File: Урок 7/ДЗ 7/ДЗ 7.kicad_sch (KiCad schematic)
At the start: 22 parts, among them SW1 SW_Push, SW2 SW_Push

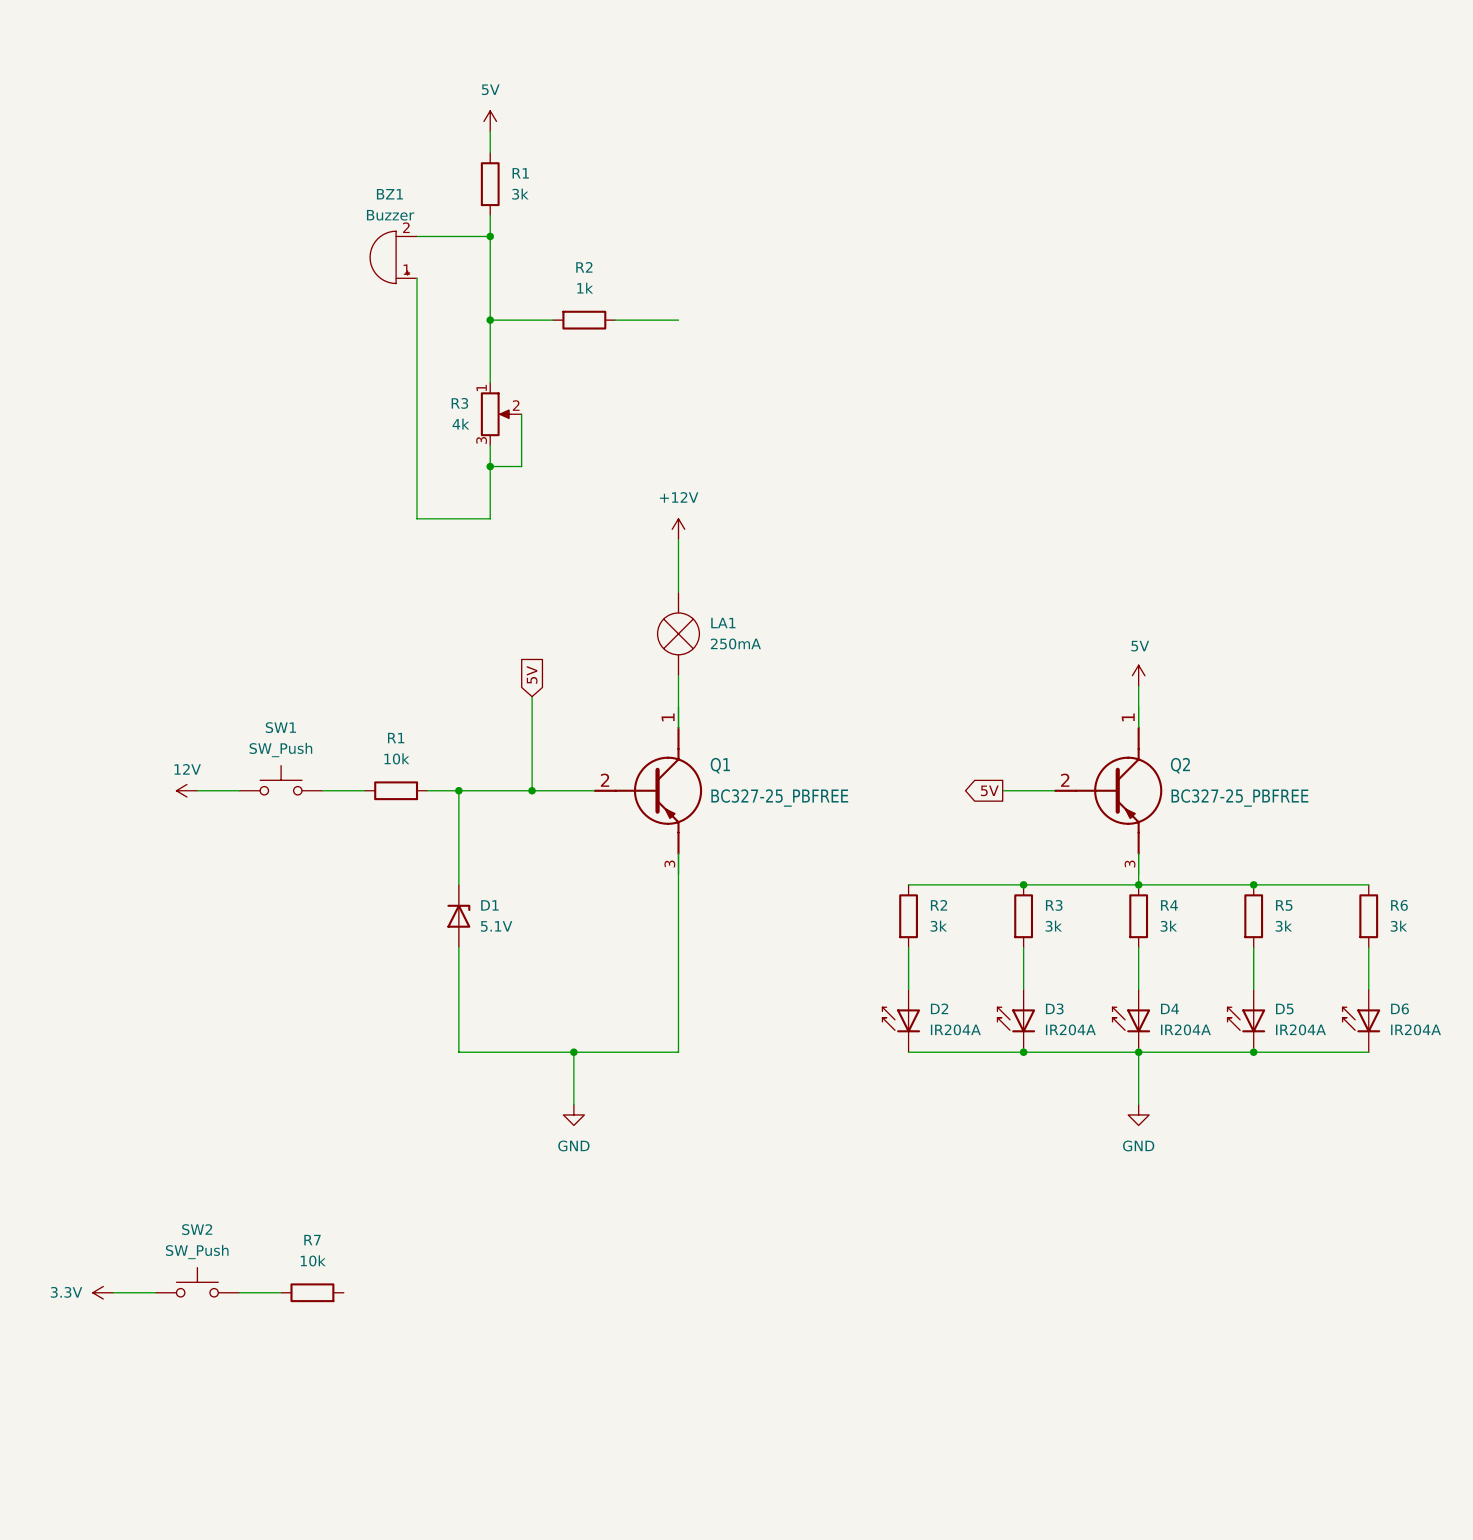
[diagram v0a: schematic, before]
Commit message: 1
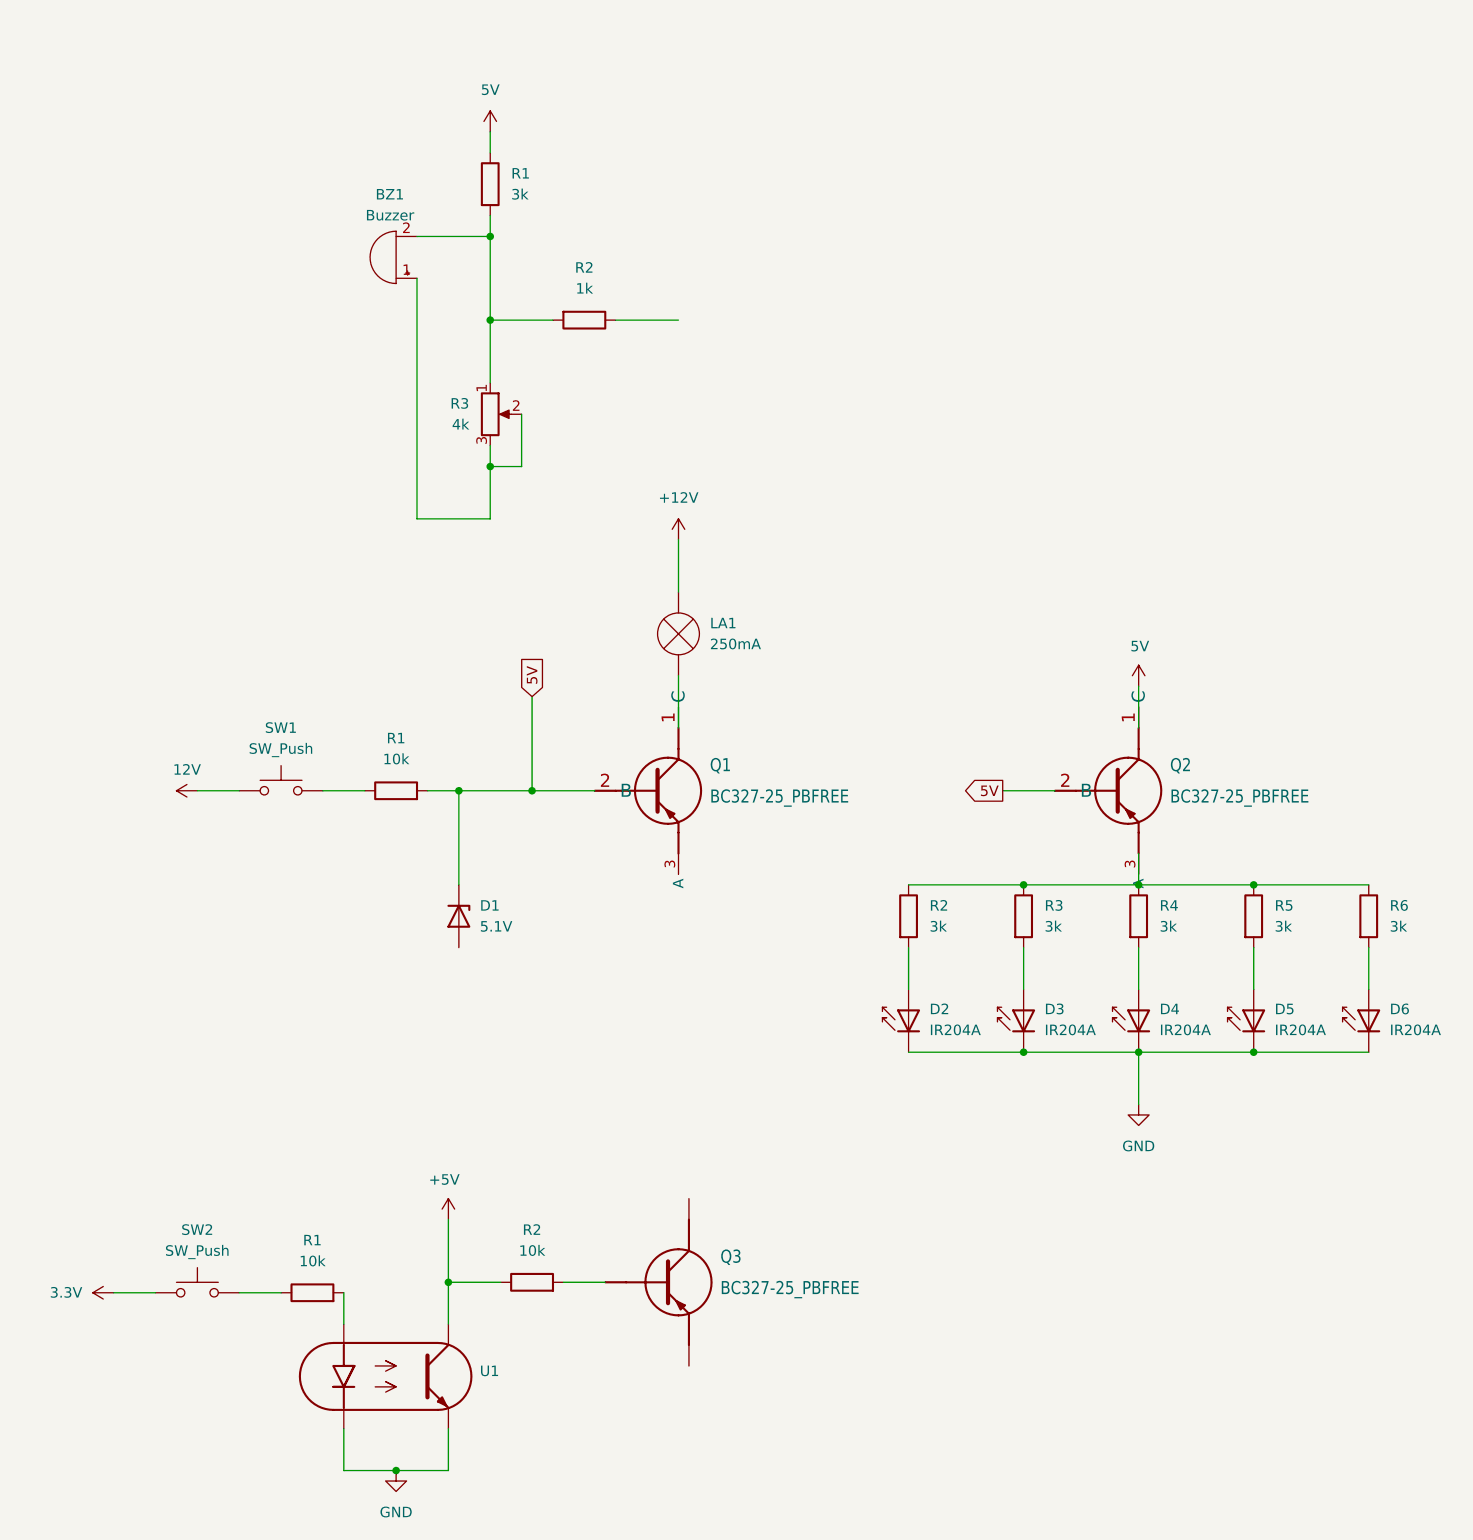
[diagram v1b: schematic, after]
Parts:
- added Q3: ~, cadstarpcblib:BC32725PBFREE, symbol My_lib2:BC327-25_PBFREE
- added R2: 10k, symbol Device:R
- added U1: ~, symbol My_lib2:PC817X3NSZ9F
- renumbered R7 to R1
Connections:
- net GND: now also U1.2 (Cathode), U1.3 (Emitter); no longer D1.2 (A), Q1.3 (A)
- net at R1.2: now also U1.1 (Anode)
- new net: Q3.2 (B), R2.2
- new net +5V: R2.1, U1.4 (Collector)

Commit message: 1
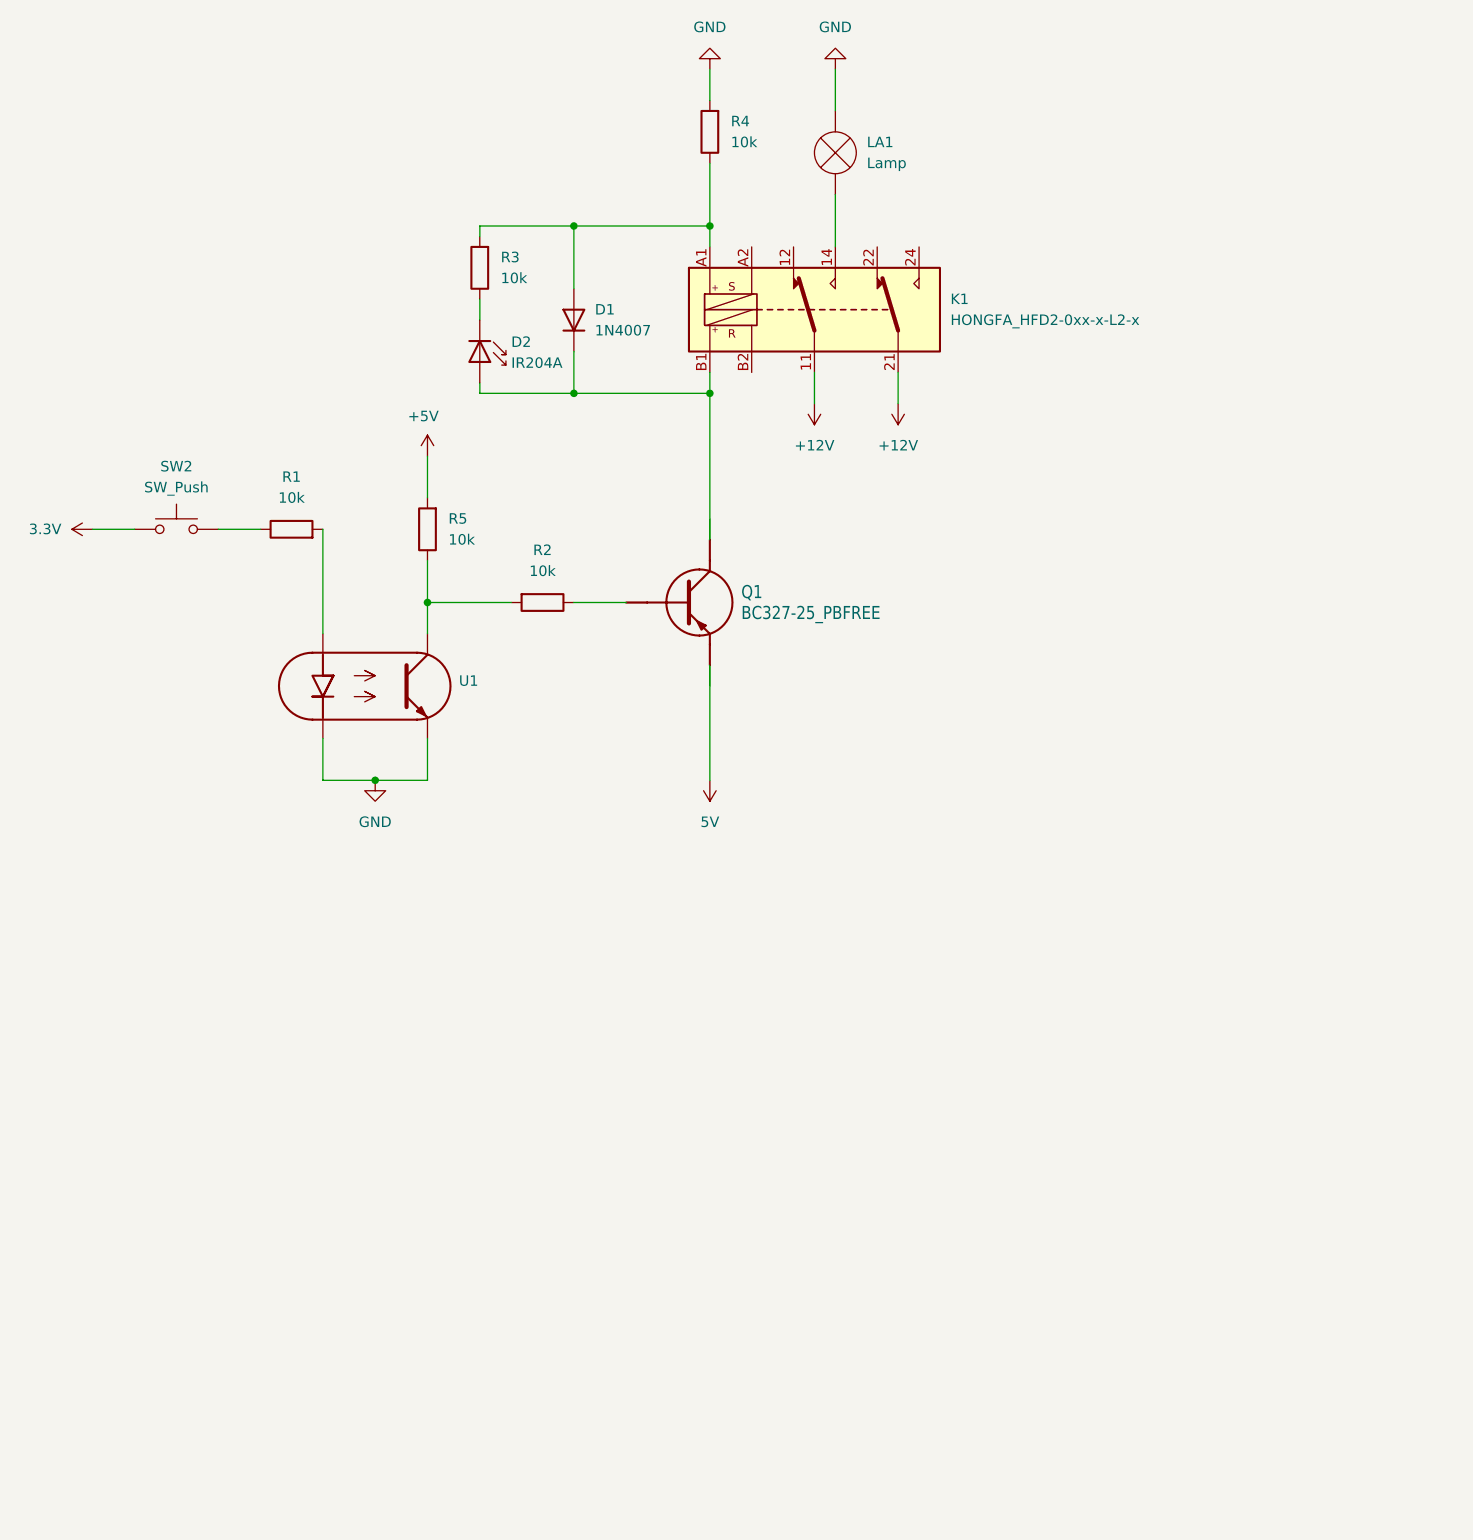
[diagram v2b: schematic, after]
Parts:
- removed BZ1: Buzzer, symbol Device:Buzzer
- removed D1: 5.1V, Diode_THT:D_DO-41_SOD81_P10.16mm_Horizontal, symbol Diode:1N47xxA
- removed D3, D4, D5, D6: IR204A, LED_THT:LED_D3.0mm_IRBlack, symbol LED:IR204A
- removed Q1, Q2: ~, cadstarpcblib:BC32725PBFREE, symbol My_lib2:BC327-25_PBFREE
- removed R1, R2: 10k, symbol Device:R
- removed R1, R2, R6: 3k, symbol Device:R
- removed R2: 1k, symbol Device:R
- removed R3: 4k, symbol Device:R_Potentiometer
- removed SW1: SW_Push, symbol Switch:SW_Push
- added D1: 1N4007, Diode_THT:D_DO-41_SOD81_P10.16mm_Horizontal, symbol Diode:1N4007
- added K1: HONGFA_HFD2-0xx-x-L2-x, Relay_THT:Relay_DPDT_Omron_G6AK, symbol Relay:HONGFA_HFD2-0xx-x-L2-x
- added R2: 10k, symbol Device:R
- LA1: value 250mA -> Lamp
- R3, R4, R5: value 3k -> 10k
- renumbered Q3 to Q1
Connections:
- net +12V: now also K1.11, K1.21; no longer LA1.2 (+)
- net +5V: now also R5.2; no longer U1.4 (Collector)
- net 5V: now also Q1.3 (A)
- net GND: now also LA1.2 (+), R4.2; no longer D2.1 (K)
- net at D2.2 (A): now also Q1.1 (C), D1.1 (K), K1.B1
- net at LA1.1 (-): now also K1.14
- net at Q1.2 (B): now also R2.1
- net at R3.2: now also R4.1, D1.2 (A), K1.A1
- new net: R2.2, R5.1, U1.4 (Collector)
- new net: D2.1 (K), R3.1
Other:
- moved on the sheet: Q1, R1, SW2, U1
